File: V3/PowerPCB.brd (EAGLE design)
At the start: 171.9 x 151.6 mm, 107 parts, among them CON2 PINHEAD_1X08-2.54-FEMALE, CON3 PINHEAD_1X08-2.54-FEMALE, CON4 PINHEAD_1X06-2.54-FEMALE, CON7 PINHEAD_1X06-2.54-FEMALE, IC1 TPS54560B, IC2 TPS54560B, IC3 TPS54560B, IC4 TPS54560B, IC5 INA169, J1 CONNECTION-7MM, M1 BATTERY_CON-XT30-RA, M2 BATTERY_CON-XT30-RA, M3 BATTERY_CON-XT30-RA, M4 BATTERY_CON-XT30-RA, M5 BATTERY_CON-XT30-RA, M6 BATTERY_CON-XT30-RA, M7 BATTERY_CON-XT30-RA, Q1 IRFR2407PBF, Q2 IRFR2407PBF, Q3 IRFR2407PBF

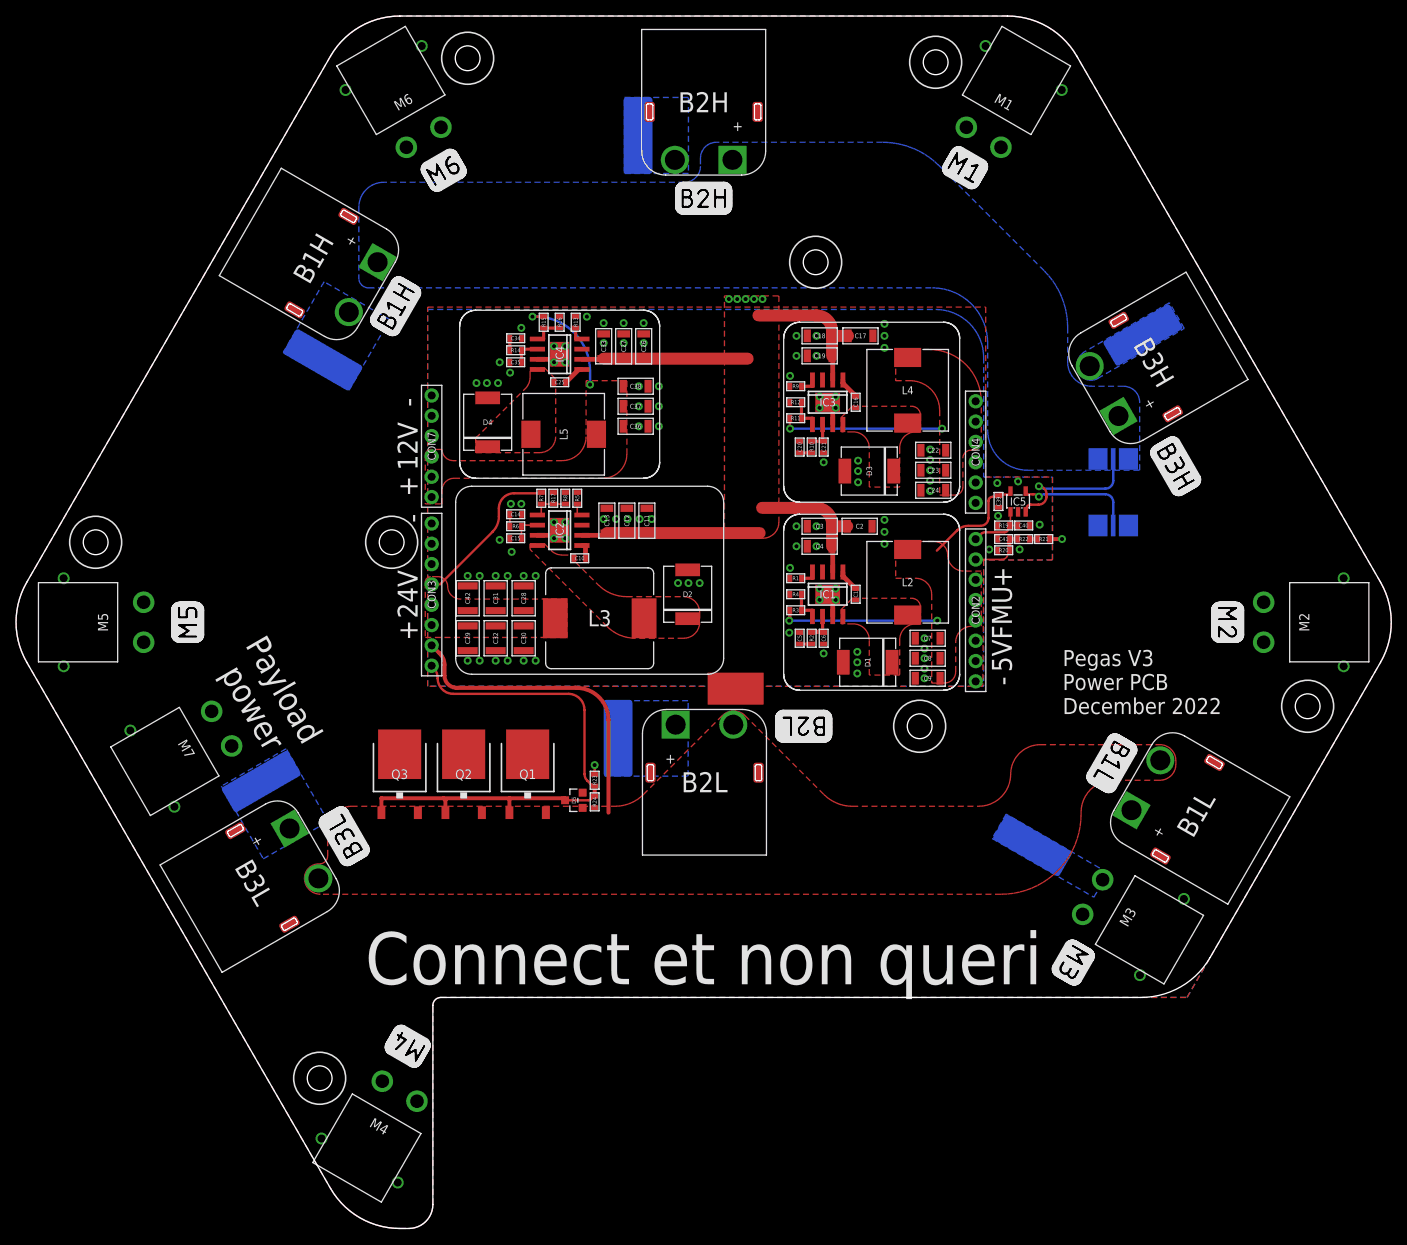
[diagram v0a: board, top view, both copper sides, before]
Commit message: updates for V3
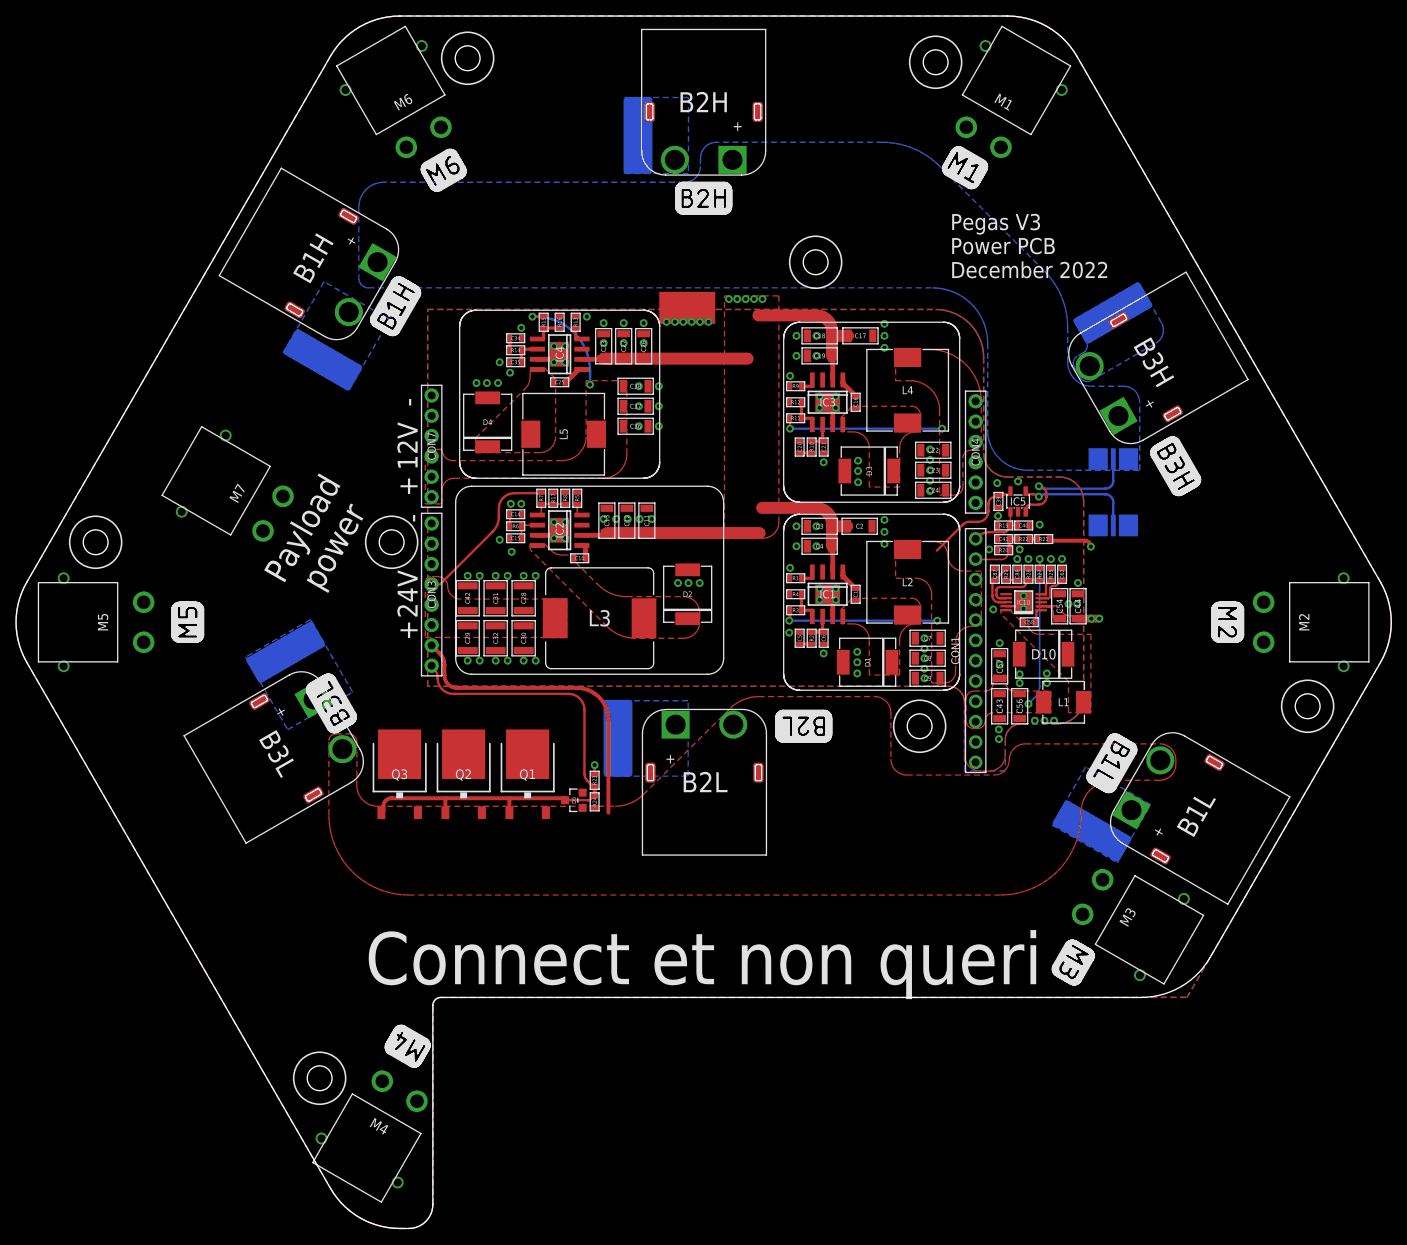
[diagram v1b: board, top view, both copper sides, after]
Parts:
- removed CON2: PINHEAD_1X08-2.54-FEMALE, pinhead:1X08-PTH-2.54-FEMALE
- added C43, C56, C57: 47u, rc:C1206
- added C44, C54: 2.2u, rc:C1206
- added C58: 0.1u, rc:C0603
- added C62: 10n, rc:C0603
- added C87: 47p, rc:C0603
- added C88: 4700p, rc:C0603
- added CON1: PINHEAD_1X12-2.54-FEMALE, pinhead:1X12-PTH-2.54-FEMALE
- added D10: B560C, Diodes:DO-214AB(SMC)
- added IC10: TPS54260, dc-dc:MSOP10
- added L1: 3.3uH, power_inductors:IHLP-2020BZ-01
- added R25, R27: 143K, rc:R0603
- added R28: 10K, rc:R0603
- added R29: 18K, rc:R0603
- moved J1 48.0 mm to (-2.05, 39.3), turned to 270 degrees
- moved M7 27.6 mm to (-53.8, 13.6), turned to 60 degrees
- moved PAD1 16.4 mm to (-52.2, -3.75)
- moved B3L 16.4 mm to (-53.2, -16.3)
- moved PAD8 7.66 mm to (48.5, -26.1)
- moved PAD2 4.65 mm to (51.1, 38.6)
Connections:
- new net BOOT: C58.2, IC10.1
- new net N$20: C62.1, IC10.4
- new net N$38: C87.1, IC10.8, R29.2
- new net N$39: IC10.5, R25.2
- new net N$50: C88.1, R29.1
- new net PH: C58.1, D10.C, IC10.10, L1.P$1
- new net VDD_4V: C43.P$1, C56.P$1, C57.P$1, CON1.3, CON1.4, L1.P$2, R27.2
- new net VSENSE: IC10.7, R27.1, R28.2
- net 5VFMU: now also CON1.10, CON1.8, CON1.9; no longer CON2.4, CON2.5, CON2.6
- net BATT_CURRENT: now also CON1.12; no longer CON2.8
- net BATT_VOLTAGE: now also CON1.11; no longer CON2.7
- net GND: now also C43.P$2, C44.P$1, C54.P$1, C56.P$2, C57.P$2, C62.2, C87.2, C88.2, CON1.1, CON1.2, CON1.5, CON1.6, CON1.7, D10.A, IC10.9, IC10.EP, R25.1, R28.1; no longer CON2.1, CON2.2, CON2.3
- net VBAT: now also C44.P$2, C54.P$2, IC10.2
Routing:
- net VDD_4V: track 0.00 -> 19.7 mm, vias 0 -> 2
- net VBAT: track 81.7 -> 90.9 mm, vias 7 -> 9
- net VSENSE: track 0.00 -> 8.11 mm
- net N$38: track 0.00 -> 6.34 mm
- net N$20: track 0.00 -> 4.07 mm
- net N$39: track 0.00 -> 2.65 mm
- net GND: track 10.2 -> 12.6 mm, vias 100 -> 127
- net BOOT: track 0.00 -> 2.17 mm
- net N$50: track 0.00 -> 1.40 mm
- net PWRSW: track 65.8 -> 64.9 mm
- net 5VFMU: track 33.5 -> 32.9 mm
- added copper zone on layer 1, net PH
- added copper zone on layer 1, net VDD_4V
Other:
- board text removed: "5VFMU"
